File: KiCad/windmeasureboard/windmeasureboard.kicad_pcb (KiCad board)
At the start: 2 copper layers, 101.2 x 73.2 mm, 28 parts, among them J1 ESQ-120-XX-X-D-XX, U1 ESP32-S2-DEVKITC-1, U2 LM1084ISX-5.0_NOPB, U3 INA229AIDGSR, U4 INA229AIDGSR, U5 INA229AIDGSR, U6 INA229AIDGSR, U7 INA229AIDGSR, U8 INA229AIDGSR, U9 INA229AIDGSR

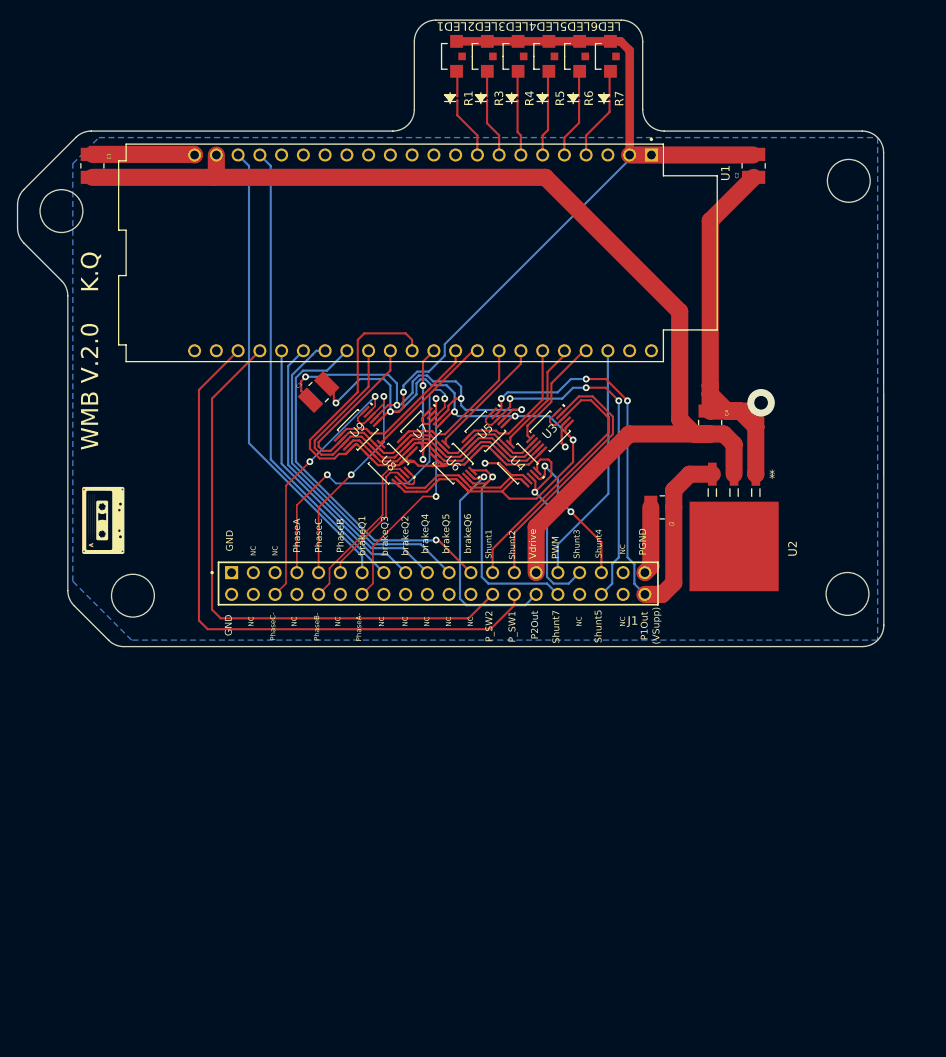
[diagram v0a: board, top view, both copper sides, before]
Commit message: Finished WMB V2.1
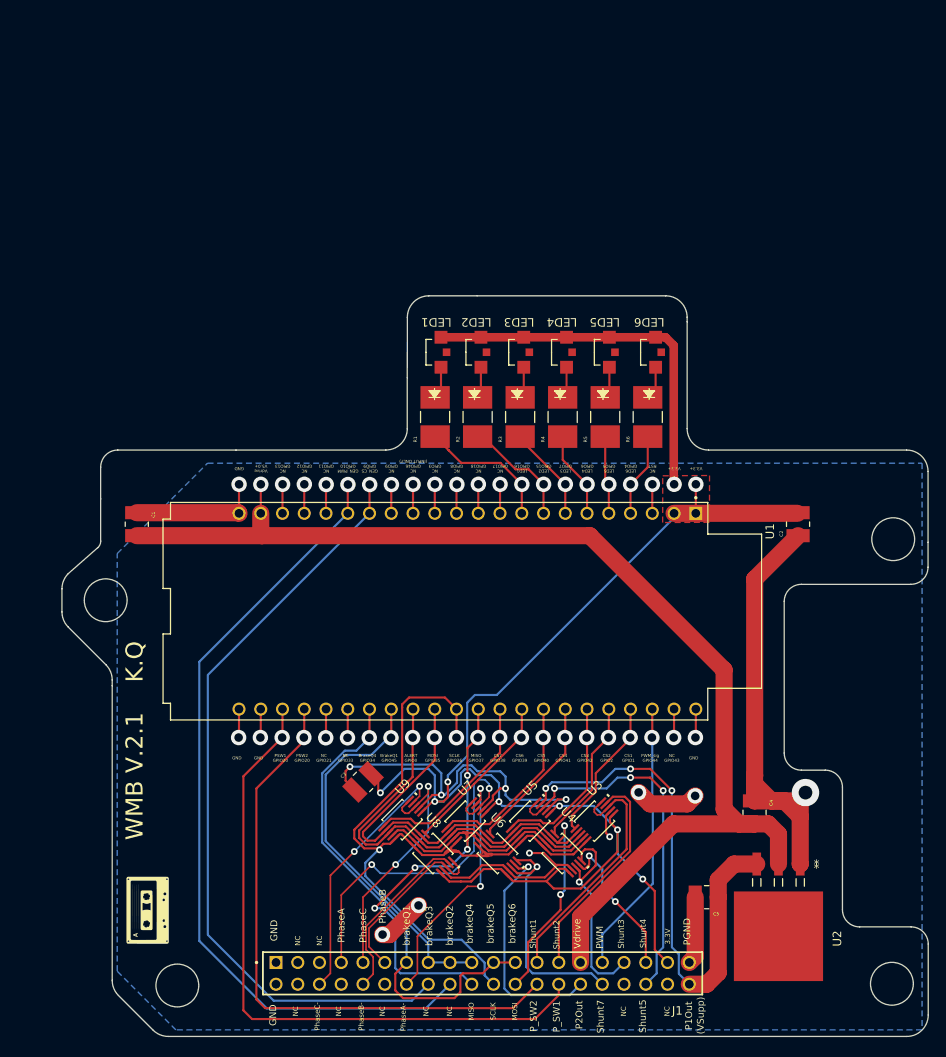
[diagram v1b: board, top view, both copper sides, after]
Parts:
- removed R7: ERJXGNJ560Y, footprints:ERJXGN_RCD
- added R2: CPA2512E56R0FS-T10, footprints:RESC6332X80N, F.Cu at (134.9, 66.7)
- R1, R3, R4, R5, R6: value ERJXGNJ560Y -> CPA2512E56R0FS-T10; footprint footprints:ERJXGN_RCD -> footprints:RESC6332X80N
- moved C5 45.8 mm to (161.6, 122.7)
- moved C3 45.8 mm to (121.5, 109.3)
- moved C4 45.8 mm to (167.2, 112.8)
- moved G*** 45.8 mm to (96.4, 124.3)
- moved J1 45.8 mm to (135.5, 131.6)
- moved U2 45.8 mm to (170.0, 127.1)
- moved U3 45.8 mm to (148.5, 113.9)
- moved U4 45.8 mm to (144.8, 117.6)
- moved U5 45.8 mm to (141.0, 113.9)
- moved U6 45.8 mm to (137.2, 117.6)
- moved U7 45.8 mm to (133.5, 113.9)
- moved U8 45.8 mm to (129.7, 117.6)
- moved U9 45.8 mm to (126.1, 113.7)
- moved C1 42.2 mm to (95.1, 79.2)
- moved C2 42.2 mm to (172.3, 79.2)
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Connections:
- J1 pad 16: unconnected-(J1-Pad16) -> GEN_CS
- J1 pad 17: Brake_Q3 -> Brake_Q1
- J1 pad 18: unconnected-(J1-Pad18) -> GEN_PWM
- J1 pad 19: Brake_Q2 -> Brake_Q1
- J1 pad 20: unconnected-(J1-Pad20) -> MISO
- J1 pad 21: Brake_Q5 -> Brake_Q4
- J1 pad 22: unconnected-(J1-Pad22) -> SCLK
- J1 pad 23: Brake_Q6 -> Brake_Q4
- J1 pad 24: unconnected-(J1-Pad24) -> MOSI
- J1 pad 37: unconnected-(J1-Pad37) -> V3.3+
- R3 pad 1: LED2 -> LED3
- R3 pad 2: Net-(LED2-Pad1) -> Net-(LED3-Pad1)
- R4 pad 1: LED3 -> LED4
- R4 pad 2: Net-(LED3-Pad1) -> Net-(LED4-Pad1)
- R5 pad 1: LED4 -> LED5
- R5 pad 2: Net-(LED4-Pad1) -> Net-(LED5-Pad1)
- R6 pad 1: LED5 -> LED6
- R6 pad 2: Net-(LED5-Pad1) -> Net-(LED6-Pad1)
- U1 pad J1_16: unconnected-(U1-GPIO10-PadJ1_16) -> GEN_CS
- U1 pad J1_17: unconnected-(U1-GPIO11-PadJ1_17) -> GEN_PWM
- U1 pad J1_19: Brake_Q1 -> unconnected-(U1-GPIO13-PadJ1_19)
- U1 pad J1_20: Brake_Q4 -> unconnected-(U1-GPIO14-PadJ1_20)
- U1 pad J3_11: /measurement chips/MISO -> MISO
- U1 pad J3_12: /measurement chips/SCLK -> SCLK
- U1 pad J3_13: /measurement chips/MOSI -> MOSI
- U1 pad J3_15: Brake_Q6 -> Brake_Q1
- U1 pad J3_16: Brake_Q5 -> Brake_Q4
- U1 pad J3_17: Brake_Q2 -> unconnected-(U1-GPIO33-PadJ3_17)
- U1 pad J3_18: Brake_Q3 -> unconnected-(U1-GPIO21-PadJ3_18)
- U3 pad 2: /measurement chips/MOSI -> MOSI
- U3 pad 4: /measurement chips/MISO -> MISO
- U3 pad 5: /measurement chips/SCLK -> SCLK
- U4 pad 2: /measurement chips/MOSI -> MOSI
- U4 pad 4: /measurement chips/MISO -> MISO
- U4 pad 5: /measurement chips/SCLK -> SCLK
- U5 pad 2: /measurement chips/MOSI -> MOSI
- U5 pad 4: /measurement chips/MISO -> MISO
- U5 pad 5: /measurement chips/SCLK -> SCLK
- U6 pad 2: /measurement chips/MOSI -> MOSI
- U6 pad 4: /measurement chips/MISO -> MISO
- U6 pad 5: /measurement chips/SCLK -> SCLK
- U7 pad 2: /measurement chips/MOSI -> MOSI
- U7 pad 4: /measurement chips/MISO -> MISO
- U7 pad 5: /measurement chips/SCLK -> SCLK
- U8 pad 2: /measurement chips/MOSI -> MOSI
- U8 pad 4: /measurement chips/MISO -> MISO
- U8 pad 5: /measurement chips/SCLK -> SCLK
- U9 pad 2: /measurement chips/MOSI -> MOSI
- U9 pad 4: /measurement chips/MISO -> MISO
- U9 pad 5: /measurement chips/SCLK -> SCLK
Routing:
- net GEN_PWM: track 0.00 -> 94.3 mm, vias 0 -> 1
- net GEN_CS: track 0.00 -> 90.2 mm, vias 0 -> 1
- net SCLK: track 0.00 -> 89.1 mm, vias 0 -> 2
- net MISO: track 0.00 -> 78.7 mm, vias 0 -> 5
- net MOSI: track 0.00 -> 72.8 mm, vias 0 -> 3
- net /measurement chips/SCLK: track 58.9 -> 0.00 mm
- net /measurement chips/MOSI: track 45.9 -> 0.00 mm
- net /measurement chips/MISO: track 43.1 -> 0.00 mm, vias 2 -> 0
- net Brake_Q6: track 42.9 -> 0.00 mm, vias 1 -> 0
- net Brake_Q5: track 39.1 -> 0.00 mm
- net V3.3+: track 174.9 -> 210.9 mm, vias 6 -> 9
- net Brake_Q2: track 35.5 -> 0.00 mm
- net Brake_Q3: track 32.9 -> 0.00 mm
- net GND: track 144.0 -> 173.8 mm, vias 7 -> 15
- net Brake_Q1: track 54.9 -> 44.8 mm, vias 0 -> 1
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- added copper zone on F.Cu, net MISO
- added copper zone on F.Cu, net SCLK
- added copper zone on F.Cu, net V3.3+
- removed copper zone on F.Cu, net /measurement chips/MISO
- removed copper zone on F.Cu, net /measurement chips/SCLK
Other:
- board size 101.2 x 73.2 mm -> 101.2 x 86.5 mm
- board text added: "3.3V"
- board text added: "ALERT GPIO0"
- board text added: "BrakeQ1 GPIO45"
- board text added: "BrakeQ4 GPIO34"
- board text added: "CS1 GPIO1"
- board text added: "CS2 GPIO2"
- board text added: "CS3 GPIO42"
- board text added: "CS4 GPIO41"
- board text added: "CS5 GPIO40"
- board text added: "CS6 GPIO39"
- board text added: "CS7 GPIO38"
- board text added: "GEN_CS GPIO9"
- board text added: "GEN_PWM GPIO10"
- board text added: "LED1 GPIO16"
- board text added: "LED2 GPIO15"
- board text added: "LED3 GPIO7"
- board text added: "LED4 GPIO6"
- board text added: "LED5 GPIO5"
- board text added: "LED6 GPIO4"
- board text added: "MISO"
- board text added: "MISO GPIO37"
- board text added: "MOSI"
- board text added: "MOSI GPIO35"
- board text added: "NC GPIO11"
- board text added: "NC GPIO12"
- board text added: "NC GPIO13"
- board text added: "NC GPIO17"
- board text added: "NC GPIO18"
- board text added: "NC GPIO21"
- board text added: "NC GPIO3"
- board text added: "NC GPIO33"
- board text added: "NC GPIO43"
- board text added: "NC GPIO46 (INPUT ONLY)"
- board text added: "NC GPIO8"
- board text added: "NC GPIO9"
- board text added: "NC RST"
- board text added: "PSW1 GPIO20"
- board text added: "PSW2 GPIO20"
- board text added: "PWM_sig GPIO44"
- board text added: "SCLK"
- board text added: "SCLK GPIO36"
- board text added: "V3.3+"
- board text added: "Vdrive V5.0+"
- board text added: "WMB V.2.1 K.Q"
- board text removed: "WMB V.2.0 K.Q"
